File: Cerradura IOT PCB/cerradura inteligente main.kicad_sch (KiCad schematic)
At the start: 12 parts, among them J1 servo, J2 boton, J3 TB_1X2, J4 teclado num 4x4, J5 Step_Down_Mini, U1 ESP32_DEVKITC

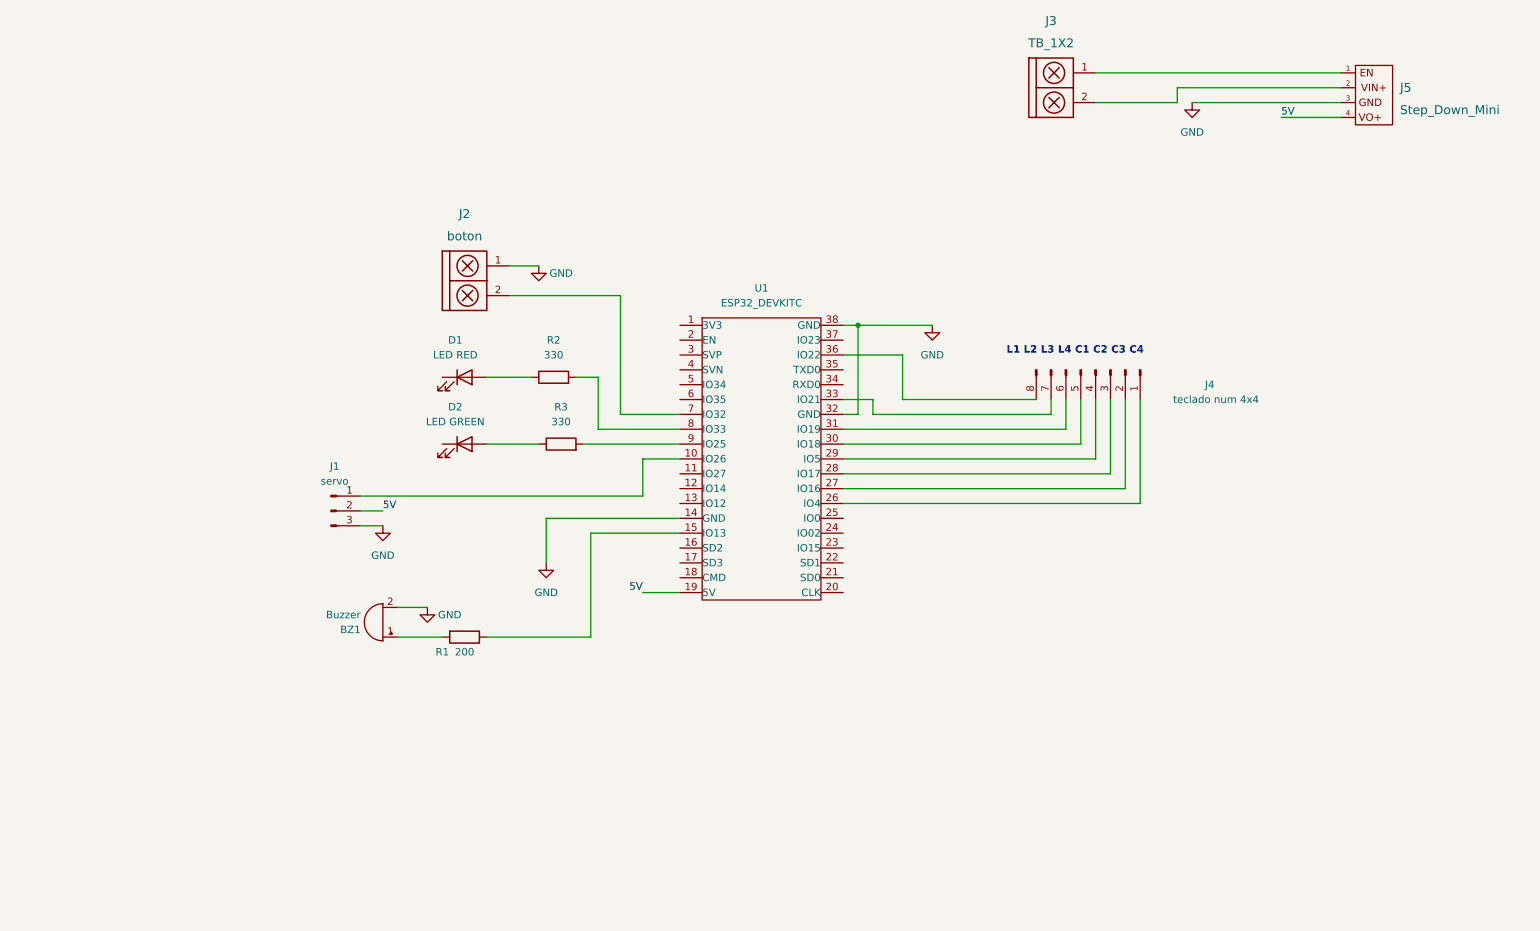
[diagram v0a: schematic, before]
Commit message: Actualizo PCB
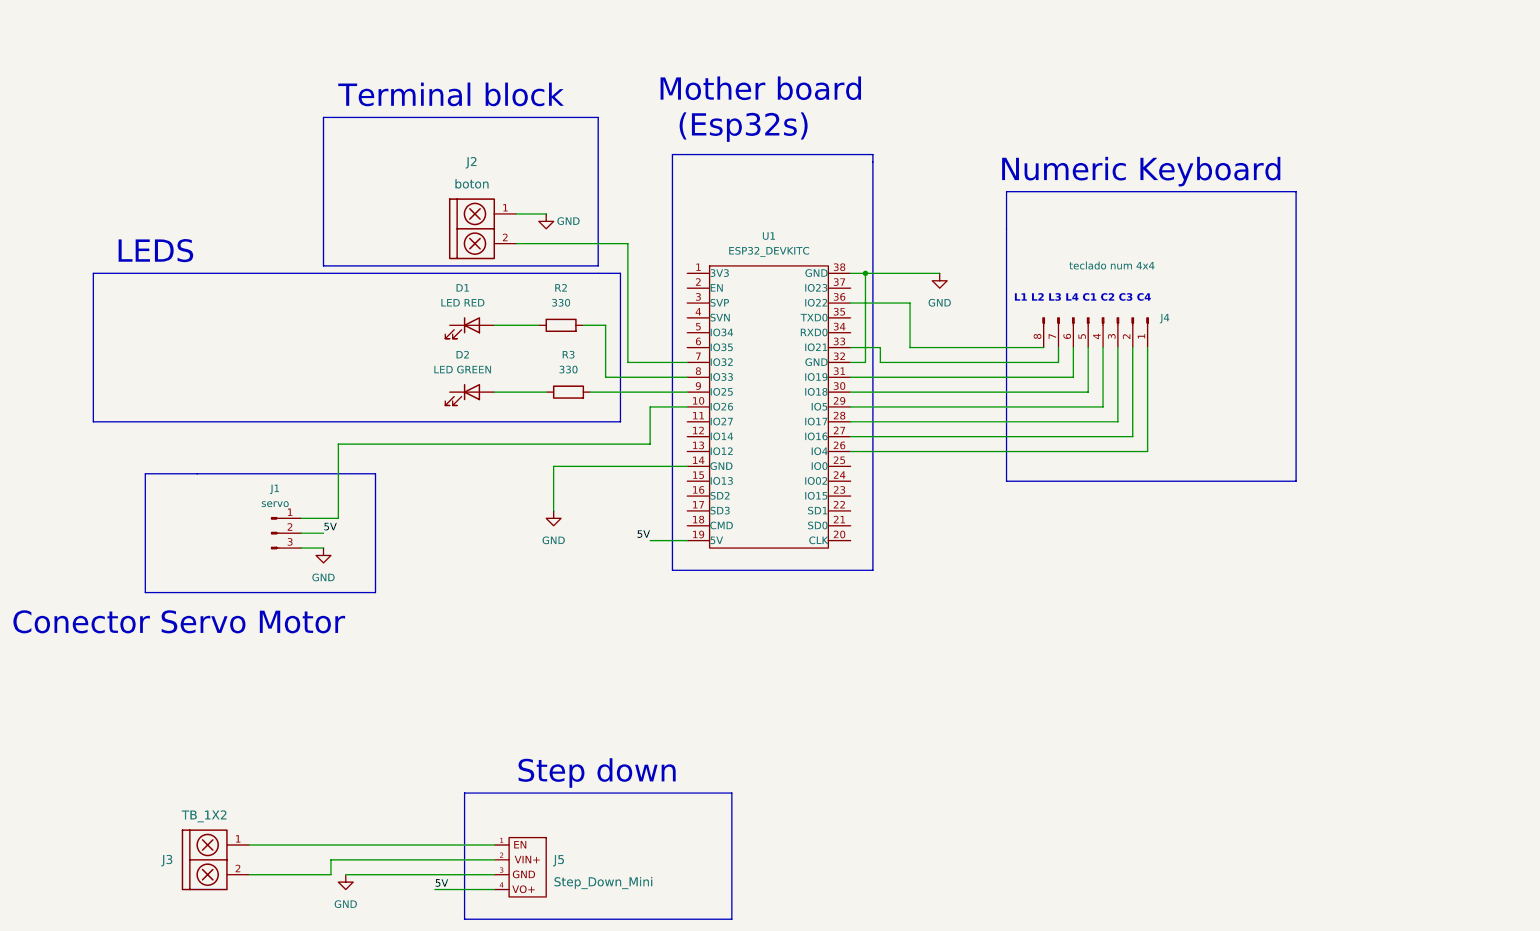
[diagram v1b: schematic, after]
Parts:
- removed BZ1: Buzzer, Buzzer_Beeper:Buzzer_Mallory_AST1109MLTRQ, symbol EESTN5:Buzzer
- removed R1: 200, EESTN5:RES0.2, symbol Device:R
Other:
- note added: "Conector Servo Motor"
- note added: "LEDS"
- note added: "Mother board (Esp32s)"
- note added: "Numeric Keyboard"
- note added: "Step down"
- note added: "Terminal block"
- company: (none) -> IHome
- title: (none) -> Electric Locker IOT
- moved on the sheet: D1, D2, J1, J2, J3, J4, J5, R2, R3, U1
